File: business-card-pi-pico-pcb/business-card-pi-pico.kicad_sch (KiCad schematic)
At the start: 48 parts, among them J1 Conn_01x04_Pin, SW1 SW_Push, U1 Pico

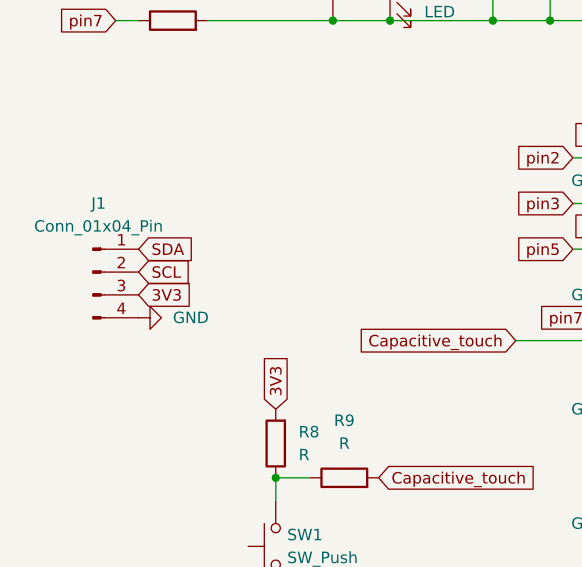
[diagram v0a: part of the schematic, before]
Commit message: backups
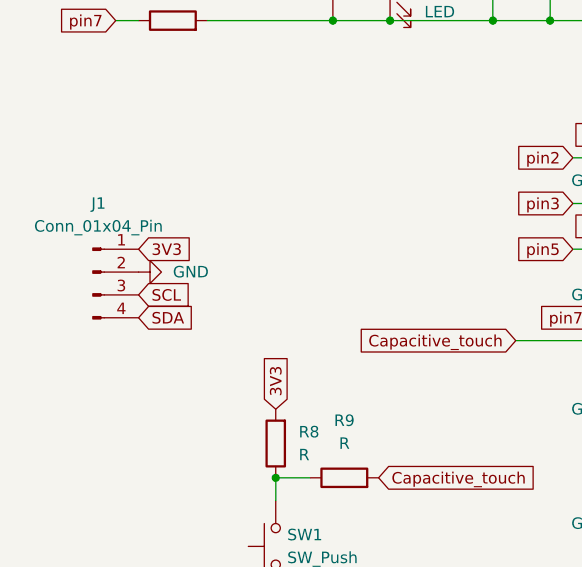
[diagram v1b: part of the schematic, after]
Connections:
- net 3V3: now also J1.1 (Pin_1); no longer J1.3 (Pin_3)
- net GND: now also J1.2 (Pin_2); no longer J1.4 (Pin_4)
- net SCL: now also J1.3 (Pin_3); no longer J1.2 (Pin_2)
- net SDA: now also J1.4 (Pin_4); no longer J1.1 (Pin_1)
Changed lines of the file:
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@@
 		)
 	)
-	(global_label "3V3"
+	(global_label "pin2"
 		(shape input)
-		(at 114.3 121.92 0)
+		(at 111.76 31.75 180)
 		(fields_autoplaced yes)
 		(effects
@@
 				(size 1.27 1.27)
 			)
-			(justify left)
+			(justify right)
 		)
 		(property "Intersheetrefs" "${INTERSHEET_REFS}"
-			(at 120.7928 121.92 0)
+			(at 104.6625 31.75 0)
 			(effects
 				(font
 					(size 1.27 1.27)
 				)
-				(justify left)
+				(justify right)
 				(hide yes)
 			)
 		)
 	)
-	(global_label "pin2"
+	(global_label "pin5"
 		(shape input)
-		(at 111.76 31.75 180)
+		(at 111.76 69.85 180)
 		(fields_autoplaced yes)
 		(effects
@@
 		)
 		(property "Intersheetrefs" "${INTERSHEET_REFS}"
-			(at 104.6625 31.75 0)
+			(at 104.6625 69.85 0)
 			(effects
 				(font
@@
 		)
 	)
-	(global_label "pin5"
+	(global_label "pin2"
 		(shape input)
-		(at 111.76 69.85 180)
+		(at 162.56 106.68 180)
 		(fields_autoplaced yes)
 		(effects
@@
 		)
 		(property "Intersheetrefs" "${INTERSHEET_REFS}"
-			(at 104.6625 69.85 0)
+			(at 155.4625 106.68 0)
 			(effects
 				(font
@@
 	(global_label "SCL"
 		(shape input)
-		(at 114.3 119.38 0)
+		(at 170.18 139.7 180)
 		(fields_autoplaced yes)
 		(effects
@@
 				(size 1.27 1.27)
 			)
-			(justify left)
+			(justify right)
 		)
 		(property "Intersheetrefs" "${INTERSHEET_REFS}"
-			(at 120.7928 119.38 0)
+			(at 163.6872 139.7 0)
 			(effects
 				(font
 					(size 1.27 1.27)
 				)
-				(justify left)
+				(justify right)
 				(hide yes)
 			)
 		)
 	)
-	(global_label "pin2"
+	(global_label "pin1"
 		(shape input)
-		(at 162.56 106.68 180)
+		(at 168.91 104.14 180)
 		(fields_autoplaced yes)
 		(effects
@@
 		)
 		(property "Intersheetrefs" "${INTERSHEET_REFS}"
-			(at 155.4625 106.68 0)
+			(at 161.8125 104.14 0)
 			(effects
 				(font
@@
 		)
 	)
-	(global_label "SCL"
+	(global_label "Capacitive_touch"
 		(shape input)
-		(at 170.18 139.7 180)
+		(at 156.21 127 180)
 		(fields_autoplaced yes)
 		(effects
@@
 		)
 		(property "Intersheetrefs" "${INTERSHEET_REFS}"
-			(at 163.6872 139.7 0)
+			(at 137.1988 127 0)
 			(effects
 				(font
@@
 		)
 	)
-	(global_label "pin1"
+	(global_label "pin4"
 		(shape input)
-		(at 168.91 104.14 180)
+		(at 111.76 57.15 180)
 		(fields_autoplaced yes)
 		(effects
@@
 		)
 		(property "Intersheetrefs" "${INTERSHEET_REFS}"
-			(at 161.8125 104.14 0)
+			(at 104.6625 57.15 0)
 			(effects
 				(font
@@
 		)
 	)
-	(global_label "Capacitive_touch"
+	(global_label "pin7"
 		(shape input)
-		(at 156.21 127 180)
+		(at 165.1 124.46 180)
 		(fields_autoplaced yes)
 		(effects
@@
 		)
 		(property "Intersheetrefs" "${INTERSHEET_REFS}"
-			(at 137.1988 127 0)
+			(at 158.0025 124.46 0)
 			(effects
 				(font
@@
 		)
 	)
-	(global_label "SDA"
+	(global_label "pin3"
 		(shape input)
-		(at 114.3 116.84 0)
+		(at 111.76 44.45 180)
 		(fields_autoplaced yes)
 		(effects
@@
 				(size 1.27 1.27)
 			)
-			(justify left)
+			(justify right)
 		)
 		(property "Intersheetrefs" "${INTERSHEET_REFS}"
-			(at 120.8533 116.84 0)
+			(at 104.6625 44.45 0)
 			(effects
 				(font
 					(size 1.27 1.27)
 				)
-				(justify left)
+				(justify right)
 				(hide yes)
 			)
 		)
 	)
-	(global_label "pin4"
+	(global_label "pin6"
 		(shape input)
-		(at 111.76 57.15 180)
+		(at 111.76 81.28 180)
 		(fields_autoplaced yes)
 		(effects
@@
 		)
 		(property "Intersheetrefs" "${INTERSHEET_REFS}"
-			(at 104.6625 57.15 0)
+			(at 104.6625 81.28 0)
 			(effects
 				(font
@@
 		)
 	)
-	(global_label "pin7"
+	(global_label "SDA"
 		(shape input)
-		(at 165.1 124.46 180)
+		(at 170.18 137.16 180)
 		(fields_autoplaced yes)
 		(effects
@@
 		)
 		(property "Intersheetrefs" "${INTERSHEET_REFS}"
-			(at 158.0025 124.46 0)
+			(at 163.6267 137.16 0)
 			(effects
 				(font
@@
 		)
 	)
-	(global_label "pin3"
+	(global_label "SDA"
 		(shape input)
-		(at 111.76 44.45 180)
+		(at 114.3 124.46 0)
 		(fields_autoplaced yes)
 		(effects
@@
 				(size 1.27 1.27)
 			)
-			(justify right)
+			(justify left)
 		)
 		(property "Intersheetrefs" "${INTERSHEET_REFS}"
-			(at 104.6625 44.45 0)
+			(at 120.8533 124.46 0)
 			(effects
 				(font
 					(size 1.27 1.27)
 				)
-				(justify right)
+				(justify left)
 				(hide yes)
 			)
@@
 	(global_label "pin6"
 		(shape input)
-		(at 111.76 81.28 180)
+		(at 170.18 119.38 180)
 		(fields_autoplaced yes)
 		(effects
@@
 		)
 		(property "Intersheetrefs" "${INTERSHEET_REFS}"
-			(at 104.6625 81.28 0)
+			(at 163.0825 119.38 0)
 			(effects
 				(font
@@
 		)
 	)
-	(global_label "SDA"
+	(global_label "3V3"
 		(shape input)
-		(at 170.18 137.16 180)
+		(at 129.54 134.62 90)
 		(fields_autoplaced yes)
 		(effects
@@
 				(size 1.27 1.27)
 			)
-			(justify right)
+			(justify left)
 		)
 		(property "Intersheetrefs" "${INTERSHEET_REFS}"
-			(at 163.6267 137.16 0)
+			(at 129.54 128.1272 90)
 			(effects
 				(font
 					(size 1.27 1.27)
 				)
-				(justify right)
+				(justify left)
 				(hide yes)
 			)
 		)
 	)
-	(global_label "pin6"
+	(global_label "pin1"
 		(shape input)
-		(at 170.18 119.38 180)
+		(at 111.76 21.59 180)
 		(fields_autoplaced yes)
 		(effects
@@
 		)
 		(property "Intersheetrefs" "${INTERSHEET_REFS}"
-			(at 163.0825 119.38 0)
+			(at 104.6625 21.59 0)
 			(effects
 				(font
@@
 		)
 	)
-	(global_label "3V3"
+	(global_label "SCL"
 		(shape input)
-		(at 129.54 134.62 90)
+		(at 114.3 121.92 0)
 		(fields_autoplaced yes)
 		(effects
@@
 		)
 		(property "Intersheetrefs" "${INTERSHEET_REFS}"
-			(at 129.54 128.1272 90)
+			(at 120.7928 121.92 0)
 			(effects
 				(font
@@
 		)
 	)
-	(global_label "pin1"
+	(global_label "3V3"
 		(shape input)
-		(at 111.76 21.59 180)
+		(at 114.3 116.84 0)
 		(fields_autoplaced yes)
 		(effects
@@
 				(size 1.27 1.27)
 			)
-			(justify right)
+			(justify left)
 		)
 		(property "Intersheetrefs" "${INTERSHEET_REFS}"
-			(at 104.6625 21.59 0)
+			(at 120.7928 116.84 0)
 			(effects
 				(font
 					(size 1.27 1.27)
 				)
-				(justify right)
+				(justify left)
 				(hide yes)
 			)
@@
 	(symbol
 		(lib_id "power:GND")
-		(at 114.3 124.46 90)
-		(unit 1)
-		(exclude_from_sim no)
-		(in_bom yes)
-		(on_board yes)
-		(dnp no)
-		(fields_autoplaced yes)
-		(property "Reference" "#PWR010"
-			(at 120.65 124.46 0)
-			(effects
-				(font
-					(size 1.27 1.27)
-				)
-				(hide yes)
-			)
-		)
-		(property "Value" "GND"
-			(at 118.11 124.4599 90)
-			(effects
-				(font
-					(size 1.27 1.27)
-				)
-				(justify right)
-			)
-		)
-		(property "Footprint" ""
-			(at 114.3 124.46 0)
-			(effects
-				(font
-					(size 1.27 1.27)
-				)
-				(hide yes)
-			)
-		)
-		(property "Datasheet" ""
-			(at 114.3 124.46 0)
-			(effects
-				(font
-					(size 1.27 1.27)
-				)
-				(hide yes)
-			)
-		)
-		(property "Description" "Power symbol creates a global label with name \"GND\" , ground"
-			(at 114.3 124.46 0)
-			(effects
-				(font
-					(size 1.27 1.27)
-				)
-				(hide yes)
-			)
-		)
-		(pin "1"
-		)
-		(instances
-			(project "business-card-pi-pico"
-				(path "/3e5122c1-1f9e-4892-9d66-f0f99c7e104b"
-					(reference "#PWR010")
-					(unit 1)
-				)
-			)
-		)
-	)
-	(symbol
-		(lib_id "power:GND")
 		(at 170.18 147.32 270)
 		(unit 1)
@@
 					(unit 1)
 				)
+			)
+		)
+	)
+	(symbol
+		(lib_id "power:GND")
+		(at 114.3 119.38 90)
+		(unit 1)
+		(exclude_from_sim no)
+		(in_bom yes)
+		(on_board yes)
+		(dnp no)
+		(fields_autoplaced yes)
+		(property "Reference" "#PWR010"
+			(at 120.65 119.38 0)
+			(effects
+				(font
+					(size 1.27 1.27)
+				)
+				(hide yes)
+			)
+		)
+		(property "Value" "GND"
+			(at 118.11 119.3799 90)
+			(effects
+				(font
+					(size 1.27 1.27)
+				)
+				(justify right)
+			)
+		)
+		(property "Footprint" ""
+			(at 114.3 119.38 0)
+			(effects
+				(font
+					(size 1.27 1.27)
+				)
+				(hide yes)
+			)
+		)
+		(property "Datasheet" ""
+			(at 114.3 119.38 0)
+			(effects
+				(font
+					(size 1.27 1.27)
+				)
+				(hide yes)
+			)
+		)
+		(property "Description" "Power symbol creates a global label with name \"GND\" , ground"
+			(at 114.3 119.38 0)
+			(effects
+				(font
+					(size 1.27 1.27)
+				)
+				(hide yes)
+			)
+		)
+		(pin "1"
+		)
+		(instances
+			(project "business-card-pi-pico"
+				(path "/3e5122c1-1f9e-4892-9d66-f0f99c7e104b"
+					(reference "#PWR010")
+					(unit 1)
+				)
